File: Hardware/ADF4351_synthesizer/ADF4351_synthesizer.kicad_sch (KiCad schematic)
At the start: 19 parts, among them J1 AVR-UPDI-6, J2 Conn_01x05_Socket, SW1 SW_Push, U1 AVR128DA32x-xPT, U6 AT24CS16-STUM

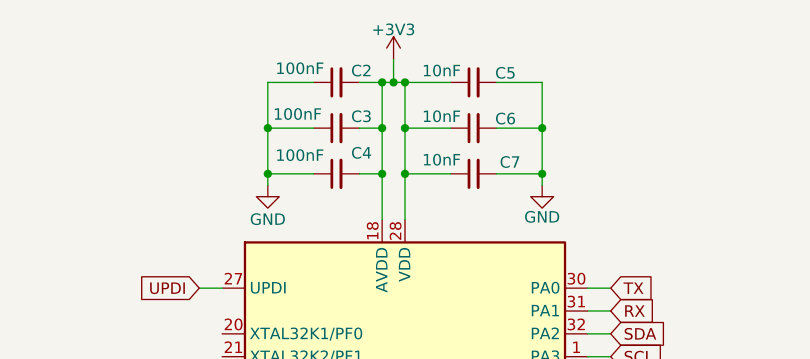
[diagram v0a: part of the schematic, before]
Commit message: Updating board
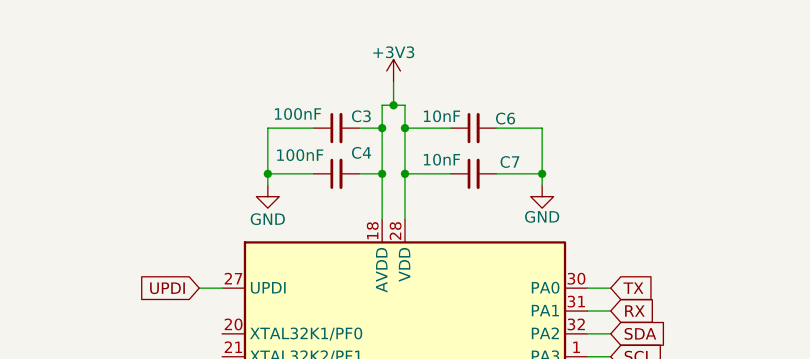
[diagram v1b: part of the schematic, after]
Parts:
- removed C2: 100nF, Capacitor_SMD:C_0402_1005Metric, symbol Device:C_Small
- removed C5: 10nF, Capacitor_SMD:C_0402_1005Metric, symbol Device:C_Small
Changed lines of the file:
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@@
 	)
 	(junction
-		(at 82.55 24.13)
-		(diameter 0)
-		(color 0 0 0 0)
-	)
-	(junction
 		(at 44.45 67.31)
 		(diameter 0)
@@
 	)
 	(junction
-		(at 100.33 29.21)
-		(diameter 0)
-		(color 0 0 0 0)
-	)
-	(junction
-		(at 69.85 29.21)
-		(diameter 0)
-		(color 0 0 0 0)
-	)
-	(junction
-		(at 83.82 24.13)
+		(at 83.82 26.67)
 		(diameter 0)
 		(color 0 0 0 0)
@@
 	)
 	(junction
-		(at 85.09 24.13)
-		(diameter 0)
-		(color 0 0 0 0)
-	)
-	(junction
 		(at 85.09 29.21)
 		(diameter 0)
@@
 	(wire
 		(pts
-			(xy 90.17 24.13) (xy 85.09 24.13)
-		)
-		(stroke
-			(width 0)
-			(type default)
-		)
-	)
-	(wire
-		(pts
 			(xy 44.45 67.31) (xy 40.64 67.31)
 		)
@@
 	(wire
 		(pts
-			(xy 82.55 29.21) (xy 82.55 34.29)
-		)
-		(stroke
-			(width 0)
-			(type default)
-		)
-	)
-	(wire
-		(pts
 			(xy 144.78 34.29) (xy 147.32 34.29)
 		)
@@
 	(wire
 		(pts
-			(xy 82.55 24.13) (xy 82.55 29.21)
+			(xy 82.55 26.67) (xy 82.55 29.21)
 		)
 		(stroke
@@
 	(wire
 		(pts
-			(xy 95.25 24.13) (xy 100.33 24.13)
-		)
-		(stroke
-			(width 0)
-			(type default)
-		)
-	)
-	(wire
-		(pts
 			(xy 105.41 161.29) (xy 105.41 160.02)
 		)
@@
 	(wire
 		(pts
-			(xy 83.82 21.59) (xy 83.82 24.13)
+			(xy 83.82 24.13) (xy 83.82 26.67)
 		)
 		(stroke
@@
 	(wire
 		(pts
-			(xy 80.01 24.13) (xy 82.55 24.13)
-		)
-		(stroke
-			(width 0)
-			(type default)
-		)
-	)
-	(wire
-		(pts
-			(xy 69.85 24.13) (xy 74.93 24.13)
-		)
-		(stroke
-			(width 0)
-			(type default)
-		)
-	)
-	(wire
-		(pts
-			(xy 100.33 24.13) (xy 100.33 29.21)
-		)
-		(stroke
-			(width 0)
-			(type default)
-		)
-	)
-	(wire
-		(pts
 			(xy 146.05 24.13) (xy 147.32 24.13)
 		)
@@
 	(wire
 		(pts
-			(xy 85.09 29.21) (xy 85.09 34.29)
-		)
-		(stroke
-			(width 0)
-			(type default)
-		)
-	)
-	(wire
-		(pts
 			(xy 105.41 69.85) (xy 107.95 69.85)
 		)
@@
 	(wire
 		(pts
-			(xy 69.85 24.13) (xy 69.85 29.21)
-		)
-		(stroke
-			(width 0)
-			(type default)
-		)
-	)
-	(wire
-		(pts
 			(xy 115.57 154.94) (xy 116.84 154.94)
 		)
@@
 	(wire
 		(pts
-			(xy 83.82 24.13) (xy 82.55 24.13)
+			(xy 83.82 26.67) (xy 82.55 26.67)
 		)
 		(stroke
@@
 	(wire
 		(pts
-			(xy 85.09 24.13) (xy 85.09 29.21)
+			(xy 82.55 29.21) (xy 82.55 34.29)
 		)
 		(stroke
@@
 	(wire
 		(pts
-			(xy 85.09 24.13) (xy 83.82 24.13)
+			(xy 85.09 26.67) (xy 85.09 29.21)
+		)
+		(stroke
+			(width 0)
+			(type default)
+		)
+	)
+	(wire
+		(pts
+			(xy 85.09 26.67) (xy 83.82 26.67)
 		)
 		(stroke
@@
 		)
 	)
+	(wire
+		(pts
+			(xy 85.09 29.21) (xy 85.09 34.29)
+		)
+		(stroke
+			(width 0)
+			(type default)
+		)
+	)
 	(text "SPI Header"
 		(exclude_from_sim no)
@@
 	)
 	(symbol
-		(lib_id "Device:C_Small")
-		(at 92.71 24.13 90)
-		(unit 1)
-		(exclude_from_sim no)
-		(in_bom yes)
-		(on_board yes)
-		(dnp no)
-		(property "Reference" "C5"
-			(at 96.266 23.114 90)
-			(effects
-				(font
-					(size 1.27 1.27)
-				)
-			)
-		)
-		(property "Value" "10nF"
-			(at 89.154 22.86 90)
-			(effects
-				(font
-					(size 1.27 1.27)
-				)
-			)
-		)
-		(property "Footprint" "Capacitor_SMD:C_0402_1005Metric"
-			(at 92.71 24.13 0)
-			(effects
-				(font
-					(size 1.27 1.27)
-				)
-				(hide yes)
-			)
-		)
-		(property "Datasheet" "~"
-			(at 92.71 24.13 0)
-			(effects
-				(font
-					(size 1.27 1.27)
-				)
-				(hide yes)
-			)
-		)
-		(property "Description" "Unpolarized capacitor, small symbol"
-			(at 92.71 24.13 0)
-			(effects
-				(font
-					(size 1.27 1.27)
-				)
-				(hide yes)
-			)
-		)
-		(pin "2"
-		)
-		(pin "1"
-		)
-		(instances
-			(project "ADF4351_synthesizer"
-				(path "/803fce22-1ef3-4294-841a-dc90f5d59ce1"
-					(reference "C5")
-					(unit 1)
-				)
-			)
-		)
-	)
-	(symbol
 		(lib_id "power:GND")
 		(at 85.09 101.6 0)
@@
 	(symbol
 		(lib_id "power:+3V3")
-		(at 83.82 21.59 0)
+		(at 83.82 24.13 0)
 		(unit 1)
 		(exclude_from_sim no)
@@
 		(dnp no)
 		(property "Reference" "#PWR05"
-			(at 83.82 25.4 0)
+			(at 83.82 27.94 0)
 			(effects
 				(font
@@
 		)
 		(property "Value" "+3V3"
-			(at 83.82 18.288 0)
+			(at 83.82 20.828 0)
 			(effects
 				(font
@@
 		)
 		(property "Footprint" ""
-			(at 83.82 21.59 0)
+			(at 83.82 24.13 0)
 			(effects
 				(font
@@
 		)
 		(property "Datasheet" ""
-			(at 83.82 21.59 0)
+			(at 83.82 24.13 0)
 			(effects
 				(font
@@
 		)
 		(property "Description" "Power symbol creates a global label with name \"+3V3\""
-			(at 83.82 21.59 0)
+			(at 83.82 24.13 0)
 			(effects
 				(font
@@
 					(unit 1)
 				)
-			)
-		)
-	)
-	(symbol
-		(lib_id "Device:C_Small")
-		(at 77.47 24.13 90)
-		(unit 1)
-		(exclude_from_sim no)
-		(in_bom yes)
-		(on_board yes)
-		(dnp no)
-		(property "Reference" "C2"
-			(at 80.264 22.86 90)
-			(effects
-				(font
-					(size 1.27 1.27)
-				)
-			)
-		)
-		(property "Value" "100nF"
-			(at 73.406 22.606 90)
-			(effects
-				(font
-					(size 1.27 1.27)
-				)
-			)
-		)
-		(property "Footprint" "Capacitor_SMD:C_0402_1005Metric"
-			(at 77.47 24.13 0)
-			(effects
-				(font
-					(size 1.27 1.27)
-				)
-				(hide yes)
-			)
-		)
-		(property "Datasheet" "~"
-			(at 77.47 24.13 0)
-			(effects
-				(font
-					(size 1.27 1.27)
-				)
-				(hide yes)
-			)
-		)
-		(property "Description" "Unpolarized capacitor, small symbol"
-			(at 77.47 24.13 0)
-			(effects
-				(font
-					(size 1.27 1.27)
-				)
-				(hide yes)
-			)
-		)
-		(pin "2"
-		)
-		(pin "1"
-		)
-		(instances
-			(project "ADF4351_synthesizer"
-				(path "/803fce22-1ef3-4294-841a-dc90f5d59ce1"
-					(reference "C2")
-					(unit 1)
-				)
